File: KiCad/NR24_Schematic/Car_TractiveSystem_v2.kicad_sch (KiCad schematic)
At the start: 12 parts, among them J1 M_con, J2 F_con, K2 Key Switch Relay, M1 Zero_7R_Motor, SW3 100V E-stop (Right), SW4 100V E-stop (Left), U1 Sevcon_Gen4_Size6, U2 Throttle, U7 Brake (AiM Pressure Sensor)

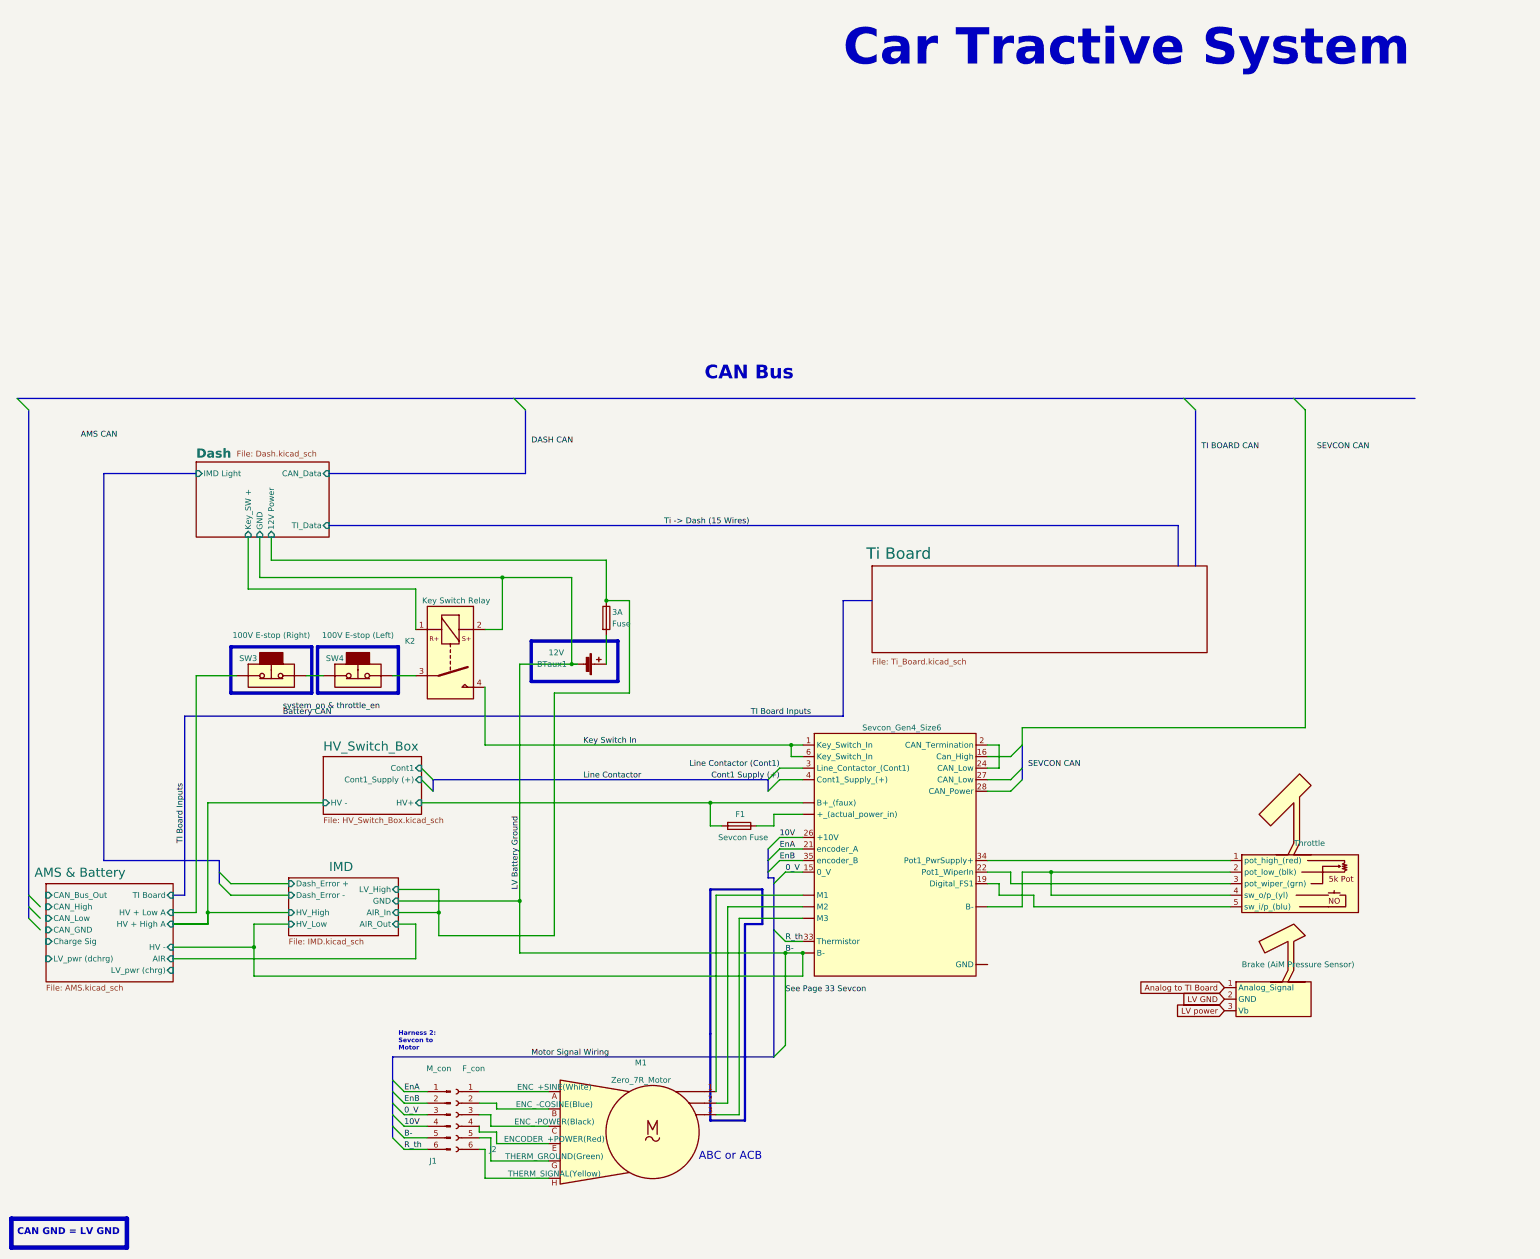
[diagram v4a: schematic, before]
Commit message: NOV1 Changes w Clarks
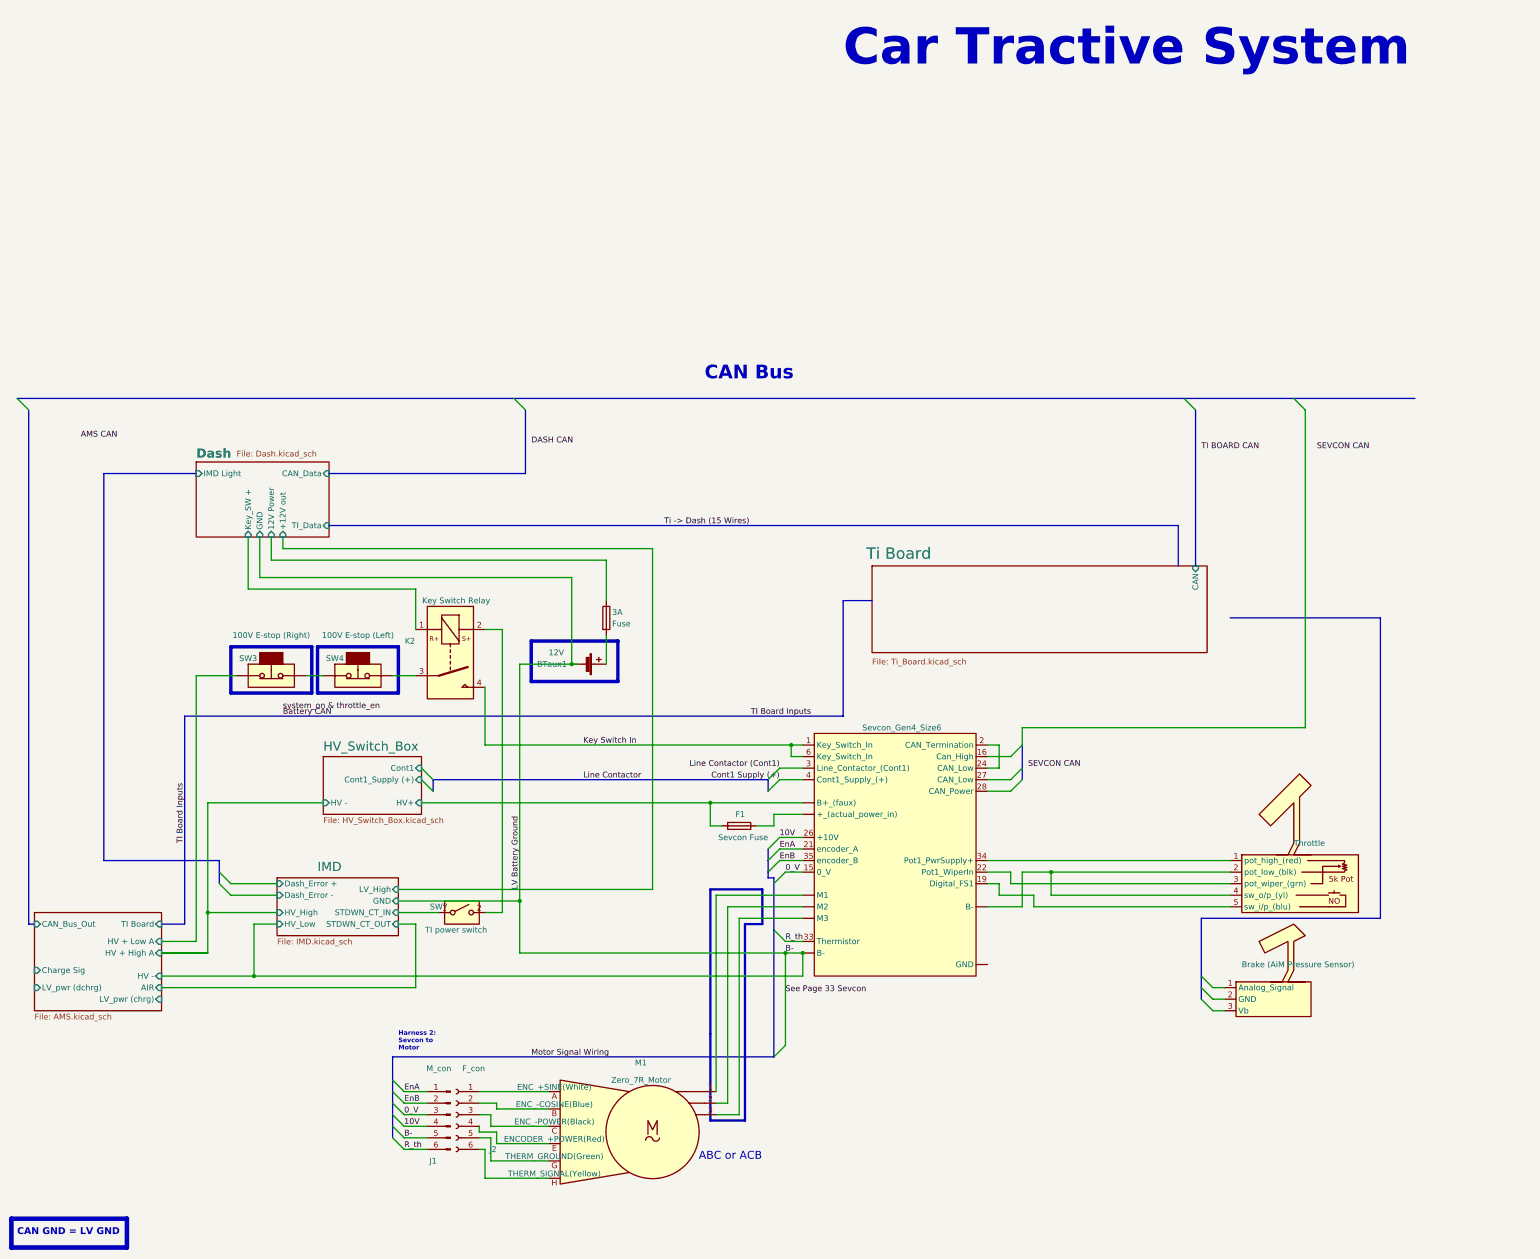
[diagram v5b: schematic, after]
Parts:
- added SW7: TI power switch, symbol CamachosSymbols:SW_SPST
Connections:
- net B-: no longer K2.2
- net  LV power: no longer names the net of U7.3 (Vb)
- net Analog to TI Board: no longer names the net of U7.1 (Analog_Signal)
- net LV GND: no longer names the net of U7.2 (GND)
- new net: K2.2, SW7.2 (B)
- new net IMD/STDWN_CT_IN: SW7.1 (A)
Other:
- sheet AMS & Battery ports: added none; removed CAN_GND, CAN_High, CAN_Low
- sheet Dash ports: added +12V out; removed none
- sheet IMD ports: added STDWN_CT_IN, STDWN_CT_OUT; removed AIR_In, AIR_Out
- sheet Ti Board ports: added CAN; removed none
